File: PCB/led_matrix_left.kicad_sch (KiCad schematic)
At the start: 42 parts

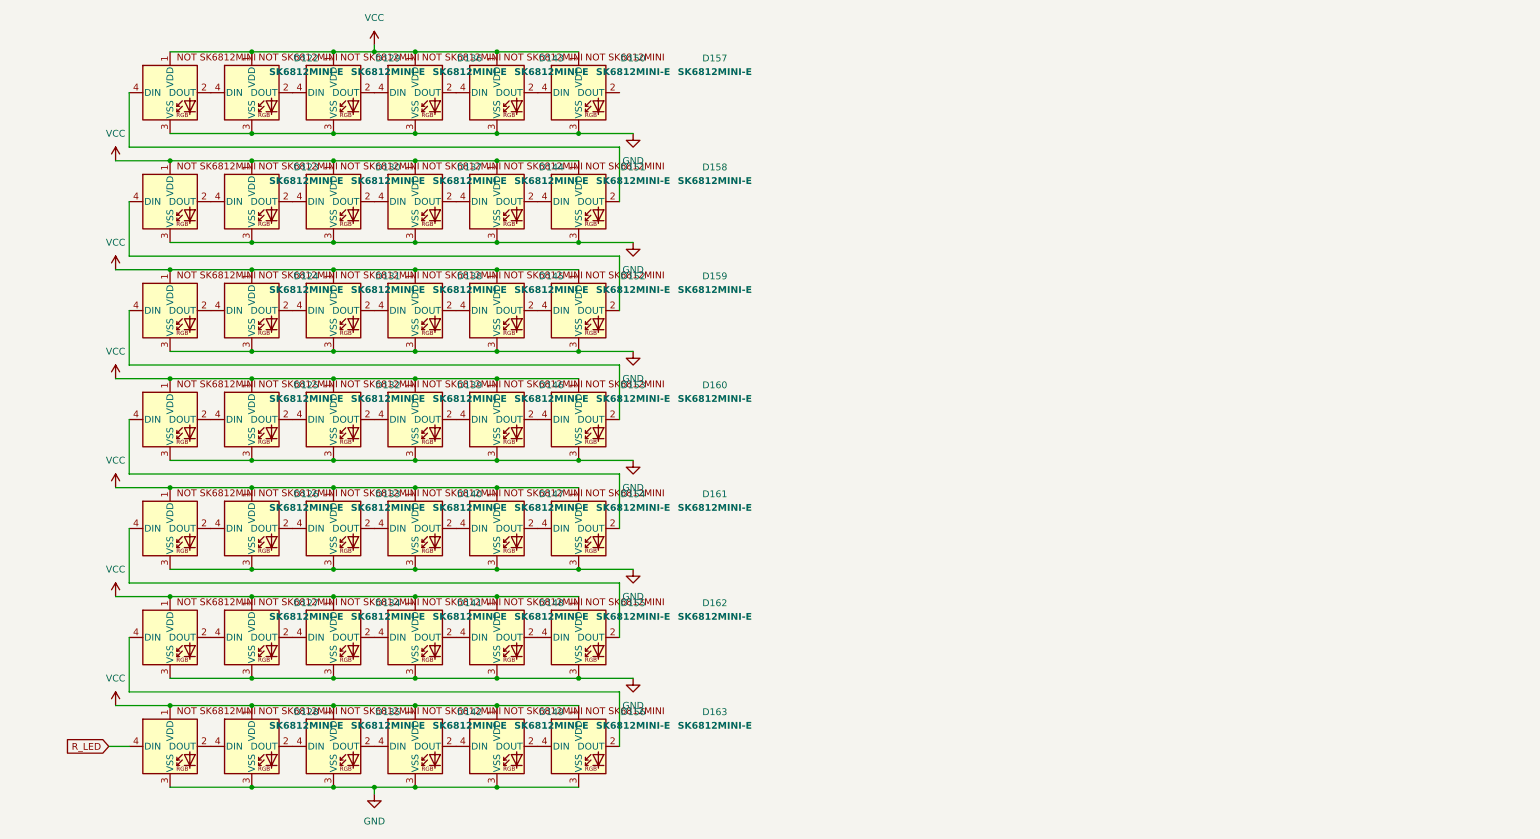
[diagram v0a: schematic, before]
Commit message: redid the leds
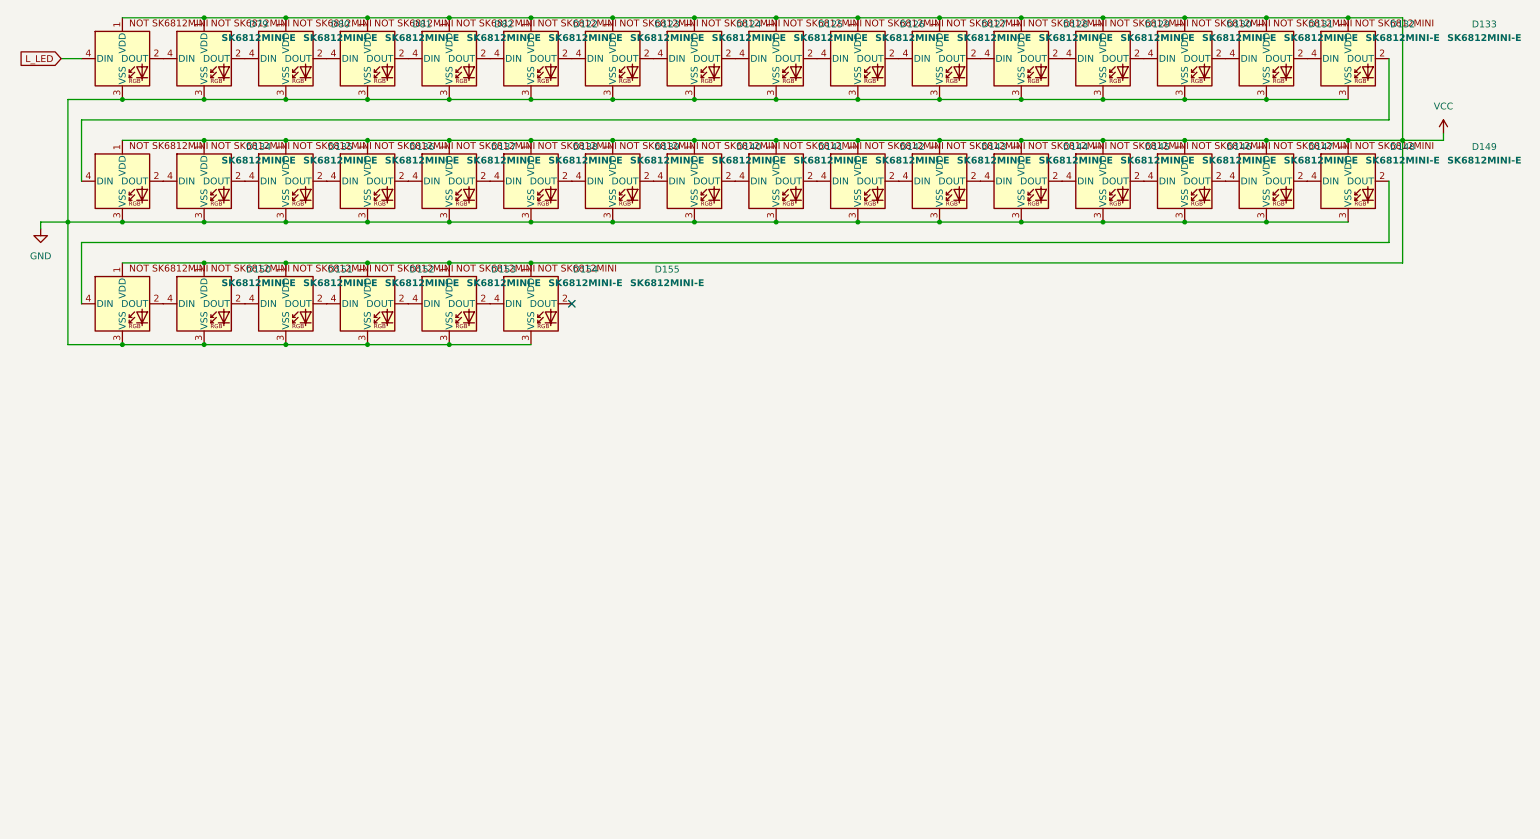
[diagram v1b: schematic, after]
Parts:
- removed D156, D157, D158, D159, D160, D161, D162, D163: SK6812MINI-E, footprints:SK6812MINI-E_fixed, symbol SK6812MINI-E:SK6812MINI-E
- added D79, D80, D81, D82: SK6812MINI-E, SK6812MINI-E - 3.2x2.8x1.78mm, symbol SK6812MINI-E:SK6812MINI-E
- D122, D123, D124, D125, D126, D127, D128, D129, D130, D131, D132, D133, D134, D135, D136, D137, D138, D139, D140, D141, D142, D143, D144, D145, D146, D147, D148, D149, D150, D151, D152, D153, D154, D155: footprint footprints:SK6812MINI-E_fixed -> SK6812MINI-E - 3.2x2.8x1.78mm
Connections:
- net R_LED is gone; now on an unnamed net: D128.4 (DIN)
- net GND: now also D79.3 (VSS), D80.3 (VSS), D81.3 (VSS), D82.3 (VSS)
- net VCC: now also D79.1 (VDD), D80.1 (VDD), D81.1 (VDD), D82.1 (VDD)
- net at D123.4 (DIN): now also D122.2 (DOUT)
- net at D152.2 (DOUT): now also D153.4 (DIN)
- net at D134.2 (DOUT): now also D135.4 (DIN); no longer D141.4 (DIN)
- net at D127.2 (DOUT): no longer D134.4 (DIN)
- net at D151.2 (DOUT): now also D152.4 (DIN)
- net at D144.2 (DOUT): now also D145.4 (DIN); no longer D151.4 (DIN)
- net at D129.4 (DIN): now also D128.2 (DOUT); no longer D122.2 (DOUT)
- net at D122.4 (DIN): now also D82.2 (DOUT)
- net at D155.4 (DIN): now also D154.2 (DOUT); no longer D148.2 (DOUT)
- net at D139.4 (DIN): now also D138.2 (DOUT); no longer D132.2 (DOUT)
- net at D132.4 (DIN): now also D131.2 (DOUT); no longer D125.2 (DOUT)
- net at D141.2 (DOUT): now also D142.4 (DIN); no longer D148.4 (DIN)
- net at D138.4 (DIN): now also D137.2 (DOUT); no longer D131.2 (DOUT)
- net at D131.4 (DIN): now also D130.2 (DOUT); no longer D124.2 (DOUT)
- net at D124.4 (DIN): now also D123.2 (DOUT)
- net at D146.4 (DIN): now also D145.2 (DOUT); no longer D139.2 (DOUT)
- net at D126.2 (DOUT): now also D127.4 (DIN); no longer D133.4 (DIN)
- net at D126.4 (DIN): now also D125.2 (DOUT)
- net at D144.4 (DIN): now also D143.2 (DOUT); no longer D137.2 (DOUT)
- net at D125.4 (DIN): now also D124.2 (DOUT)
- net at D137.4 (DIN): now also D136.2 (DOUT); no longer D130.2 (DOUT)
- net at D130.4 (DIN): now also D129.2 (DOUT); no longer D123.2 (DOUT)
- net at D153.2 (DOUT): now also D154.4 (DIN)
- net at D146.2 (DOUT): now also D147.4 (DIN); no longer D153.4 (DIN)
- net at D149.2 (DOUT): now also D150.4 (DIN)
- net at D147.2 (DOUT): now also D148.4 (DIN); no longer D154.4 (DIN)
- net at D140.2 (DOUT): now also D141.4 (DIN); no longer D147.4 (DIN)
- net at D136.4 (DIN): now also D135.2 (DOUT); no longer D129.2 (DOUT)
- net at D142.2 (DOUT): now also D143.4 (DIN); no longer D149.4 (DIN)
- net at D133.2 (DOUT): now also D134.4 (DIN); no longer D140.4 (DIN)
- net at D150.2 (DOUT): now also D151.4 (DIN)
- new net: D79.2 (DOUT), D80.4 (DIN)
- new net: D81.2 (DOUT), D82.4 (DIN)
- new net: D80.2 (DOUT), D81.4 (DIN)
- new net: D132.2 (DOUT), D133.4 (DIN)
- new net: D148.2 (DOUT), D149.4 (DIN)
- new net: D139.2 (DOUT), D140.4 (DIN)
- new net L_LED: D79.4 (DIN)
- no-connect marks 0 -> 1
